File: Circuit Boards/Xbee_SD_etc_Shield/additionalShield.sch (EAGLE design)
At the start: 52 parts, among them P1 DF3A-2P-2DSA, P2 DF3A-2P-2DSA, Q1 BSS123, Q2 BSS123, Q3 BSS123, U2 XBEE-1B3, U3 V_REG_LDOSMD, U4 V_REG_LDOSMD, U5 MAX232SOIC16, U6 ARDUINO-MEGAFULL

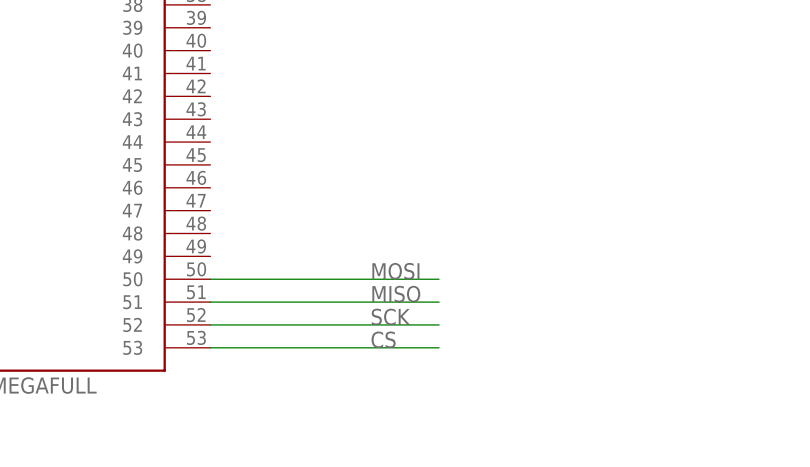
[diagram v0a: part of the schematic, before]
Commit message: got code working again
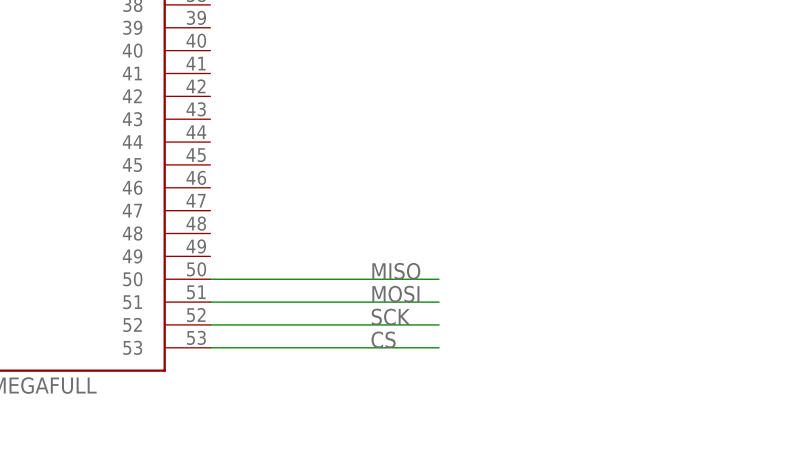
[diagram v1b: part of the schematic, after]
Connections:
- net MISO: now also U6.50; no longer U6.51
- net MOSI: now also U6.51; no longer U6.50
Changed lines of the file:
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@@
 </segment>
 <segment>
-<pinref part="U6" gate="G$1" pin="50"/>
-<wire x1="66.04" y1="-38.1" x2="91.44" y2="-38.1" width="0.1524" layer="91"/>
-<label x="83.82" y="-38.1" size="1.778" layer="95"/>
+<pinref part="U6" gate="G$1" pin="51"/>
+<wire x1="66.04" y1="-40.64" x2="91.44" y2="-40.64" width="0.1524" layer="91"/>
+<label x="83.82" y="-40.64" size="1.778" layer="95"/>
 </segment>
 </net>
@@
 </segment>
 <segment>
-<pinref part="U6" gate="G$1" pin="51"/>
-<wire x1="66.04" y1="-40.64" x2="91.44" y2="-40.64" width="0.1524" layer="91"/>
-<label x="83.82" y="-40.64" size="1.778" layer="95"/>
+<pinref part="U6" gate="G$1" pin="50"/>
+<wire x1="66.04" y1="-38.1" x2="91.44" y2="-38.1" width="0.1524" layer="91"/>
+<label x="83.82" y="-38.1" size="1.778" layer="95"/>
 </segment>
 </net>
